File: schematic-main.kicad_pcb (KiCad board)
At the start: 2 copper layers, 102.3 x 135.4 mm, 123 parts, among them IC1 AD8544ARUZ-REEL, IC2 LM76202QPWPRQ1, J1 Battery, J2 CAN, J3 V_P, J4 Conn_01x04, J6 MOTOR_DRIVER, J7 C_P, J8 VALVE, J9 PURGE_VALVE, P1 USB_C_Plug_USB2.0, U2 TPS62933, U3 USBLC6-2P6, U4 ESP32-S3FN8, U5 SN65HVD232, U6 DRV8801PWP, Y1 Crystal_GND24

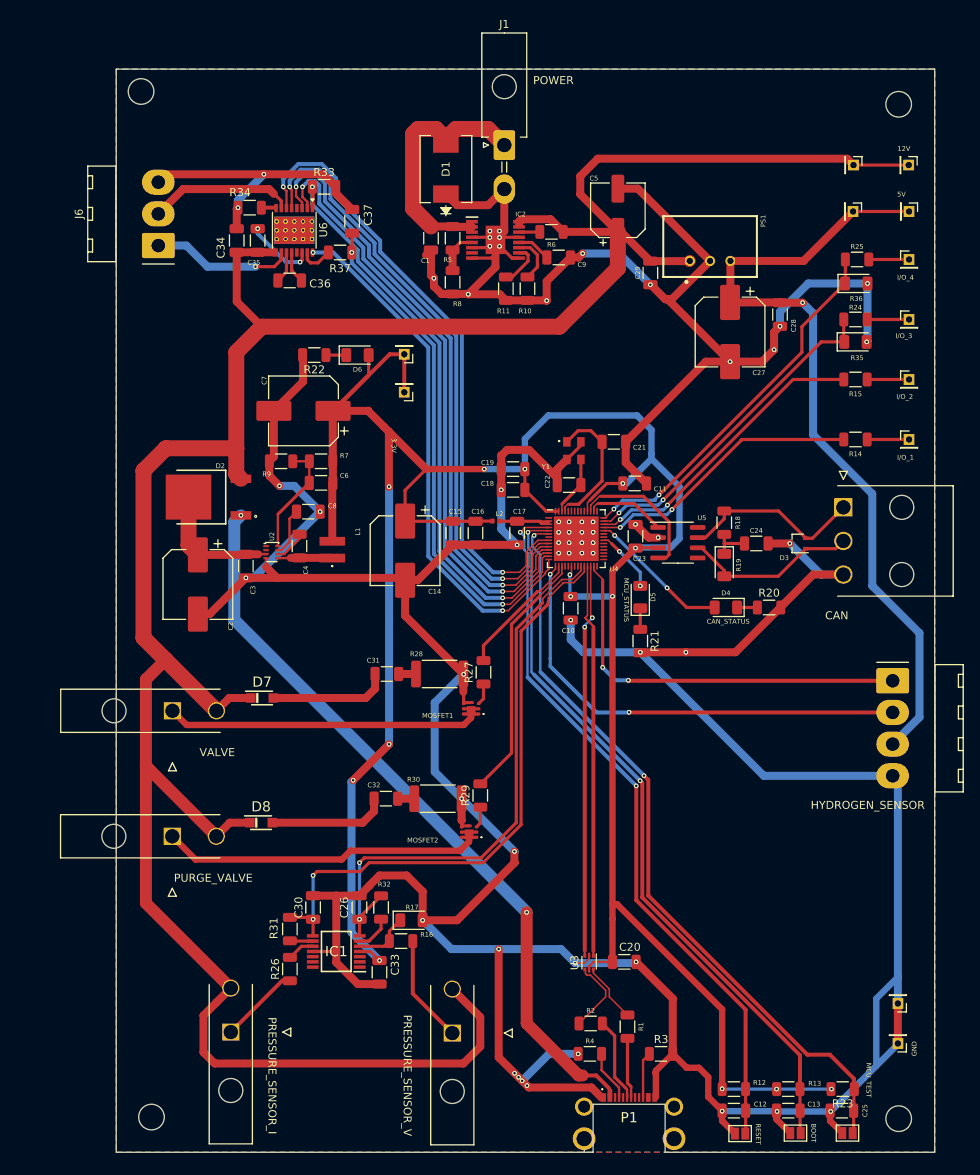
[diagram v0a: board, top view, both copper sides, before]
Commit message: Change of dimensions
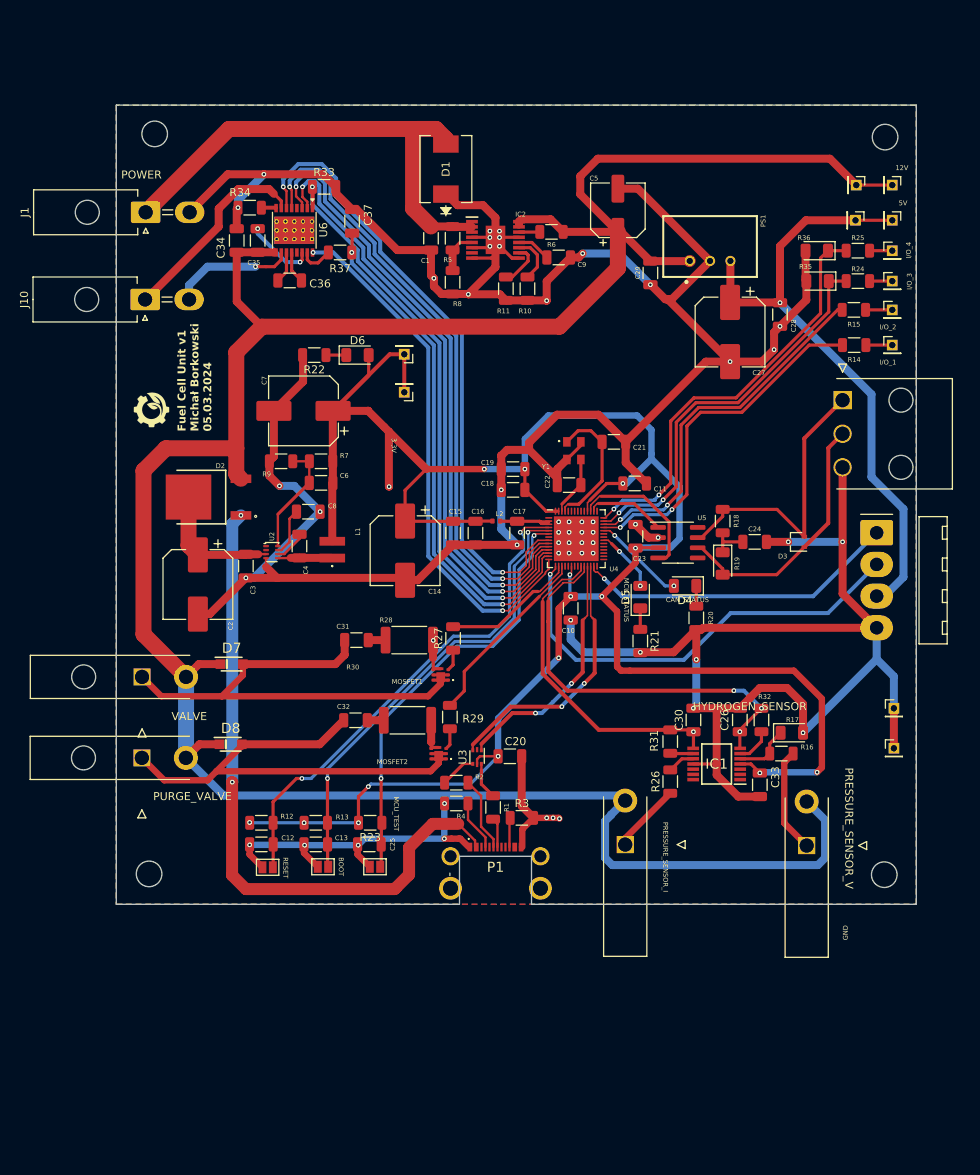
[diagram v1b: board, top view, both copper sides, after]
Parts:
- removed J6: MOTOR_DRIVER, Connector_Molex:Molex_KK-396_A-41792-0003_1x03_P3.96mm_Horizontal
- added J10: Motor, Connector_Molex:Molex_Mini-Fit_Jr_5569-02A2_2x01_P4.20mm_Horizontal, F.Cu at (52.6, 76.2)
- moved JP1 67.8 mm to (67.9, 147.2)
- moved C12 67.8 mm to (67.1, 144.3)
- moved C13 67.8 mm to (73.9, 144.3)
- moved JP2 67.8 mm to (74.8, 147.1)
- moved JP3 67.8 mm to (81.3, 147.1)
- moved R12 67.8 mm to (67.1, 141.6)
- moved R13 67.8 mm to (73.9, 141.6)
- moved R23 67.8 mm to (80.7, 141.6)
- moved C25 67.8 mm to (80.6, 144.3)
- moved J7 54.6 mm to (112.6, 144.3)
- moved C30 53.0 mm to (121.1, 128.8)
- moved C33 53.0 mm to (129.4, 136.9)
- moved R16 53.0 mm to (132.1, 133.0)
- moved R17 53.0 mm to (133.4, 130.4)
- moved R26 53.0 mm to (118.2, 136.5)
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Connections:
- C31 pad 1: Net-(D7-A) -> /IO/VALVE
- C32 pad 1: Net-(D8-A) -> /IO/PURGE_VALVE
- D7 pad 2: Net-(D7-A) -> /IO/VALVE
- D8 pad 2: Net-(D8-A) -> /IO/PURGE_VALVE
- U4 pad 23: /PRESSURE_SENSOR_V_MCU -> /PRESSURE_SENSOR_I_MCU
- U4 pad 24: /PRESSURE_SENSOR_I_MCU -> /PRESSURE_SENSOR_V_MCU
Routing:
- net GND: track 700.5 -> 551.9 mm, vias 60 -> 55
- net /MCU/MCU_TEST: track 95.1 -> 54.0 mm
- net +3.3V: track 333.6 -> 295.0 mm, vias 14 -> 16
- net /PRESSURE_SENSOR_I_MCU: track 75.5 -> 40.2 mm, vias 2 -> 1
- net /MCU/BOOT: track 91.9 -> 57.6 mm
- net /Power /Vin: track 33.1 -> 65.1 mm
- net /MCU/RESET: track 90.7 -> 62.6 mm
- net +5V: track 101.8 -> 78.9 mm
- net /MCU/USB_D-: track 56.7 -> 35.3 mm, vias 0 -> 2
- net /MCU/USB_D+: track 58.7 -> 37.9 mm
- net /IO/VALVE: track 43.5 -> 64.2 mm
- net /PRESSURE_SENSOR_V_MCU: track 71.1 -> 50.5 mm, vias 2 -> 3
- net /IO/PURGE_VALVE: track 44.4 -> 63.0 mm
- net Net-(D7-A): track 15.0 -> 0.00 mm
- net Net-(D8-A): track 14.9 -> 0.00 mm
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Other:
- board size 102.3 x 135.4 mm -> 100 x 99.9 mm
- board text added: "Fuel Cell Unit v1 Michał Borkowski 05.03.2024"
- board text removed: "CAN"
